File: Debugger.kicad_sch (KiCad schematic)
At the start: 33 parts, among them J4 F103 SWD, J5 USB_B_Micro, SW5 SW_Push, U3 STM32F103C8T6, U4 USBLC6-2, Y1 8MHz

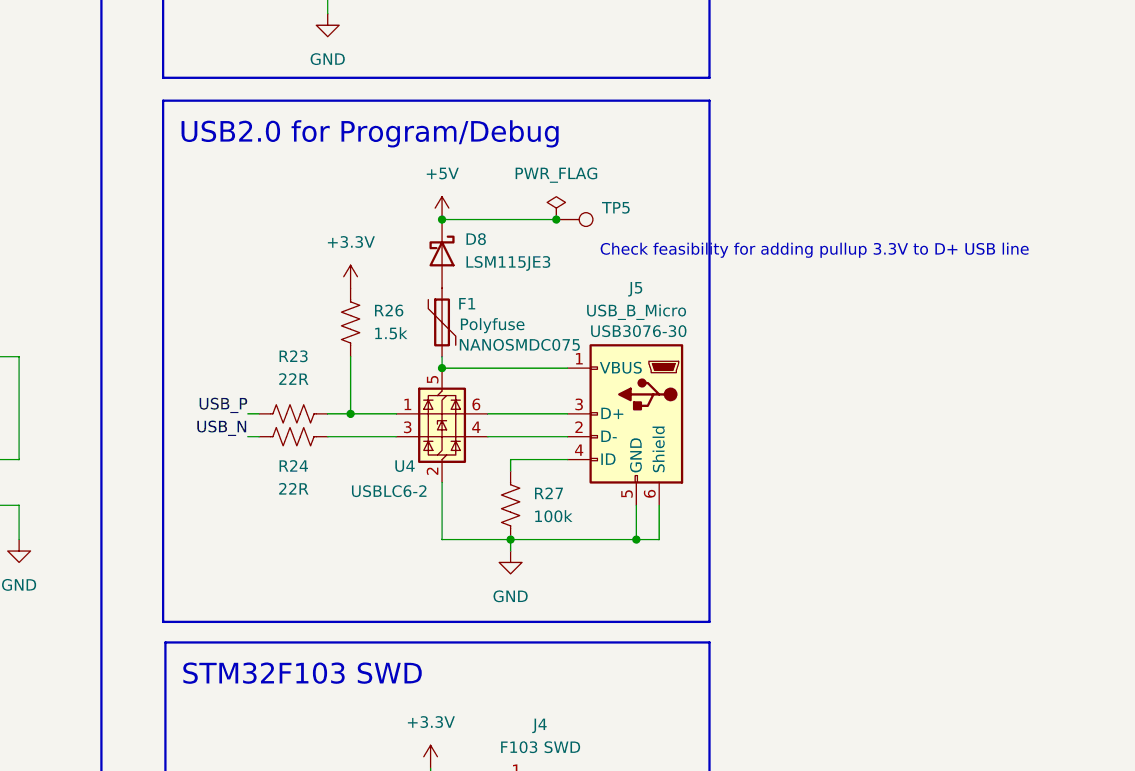
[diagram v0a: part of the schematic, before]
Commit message: All comments addressed
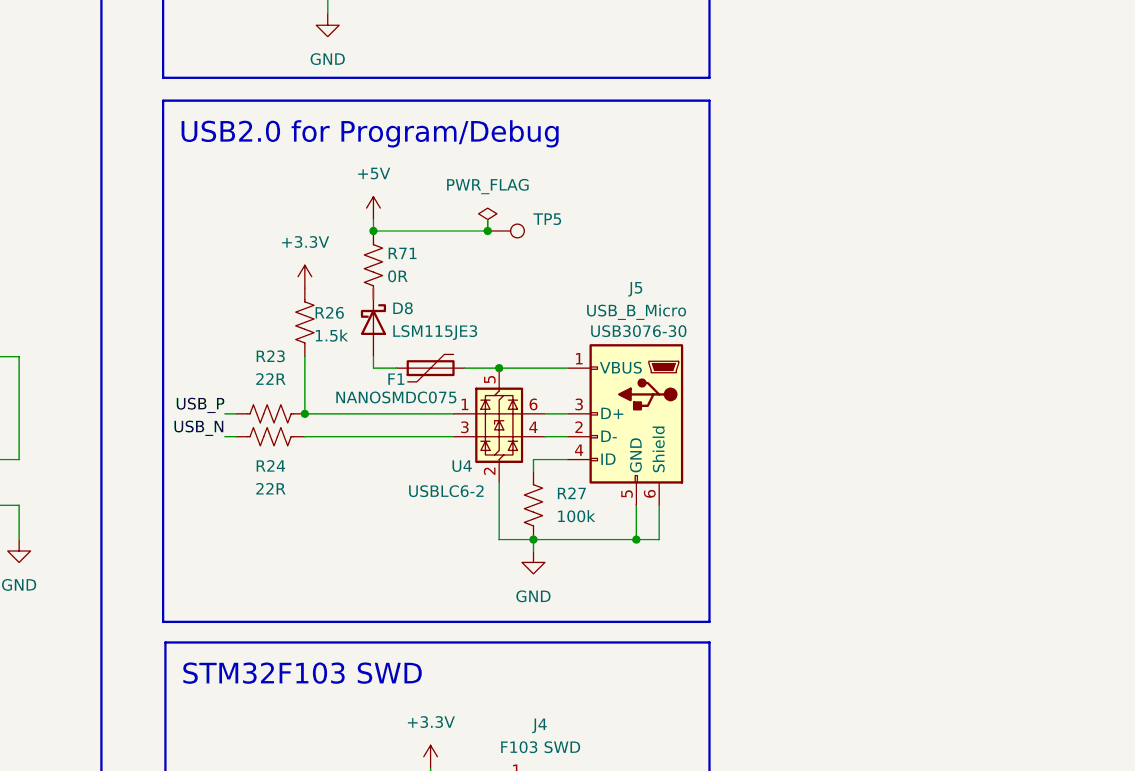
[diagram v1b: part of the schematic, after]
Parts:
- added R71: 0R, Resistor_SMD:R_0603_1608Metric, symbol Device:R_US
- SW5: MPN PTS645SK50SMTR92 LFS -> SWT0310-043016GSA
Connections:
- net +5V: now also R71.2; no longer D8.1 (K)
- new net: D8.1 (K), R71.1
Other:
- note removed: "Check feasibility for adding pullup 3.3V to D+ USB line"
- moved on the sheet: D8, F1, R23, R24, R26, R27, TP5, U4
